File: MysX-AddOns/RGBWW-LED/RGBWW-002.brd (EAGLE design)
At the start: 47 x 53 mm, 14 parts

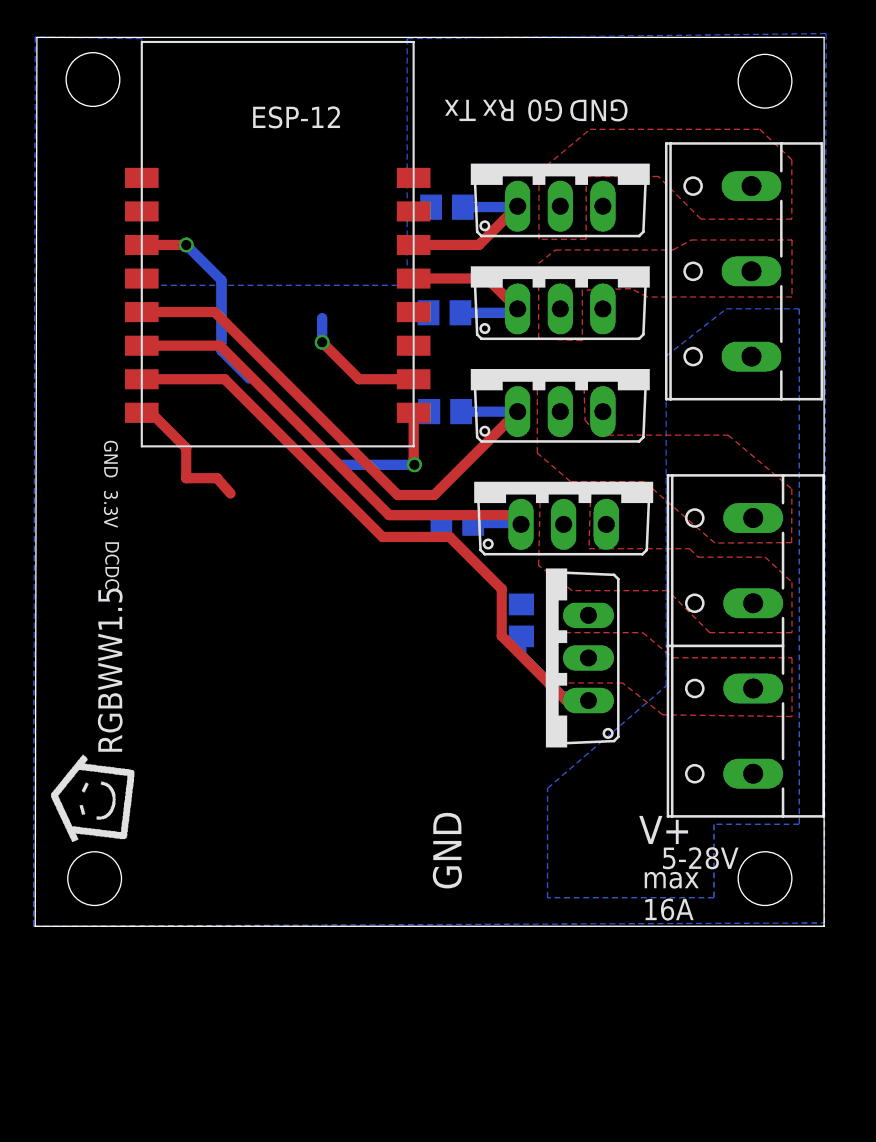
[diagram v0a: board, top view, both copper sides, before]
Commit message: AddOns
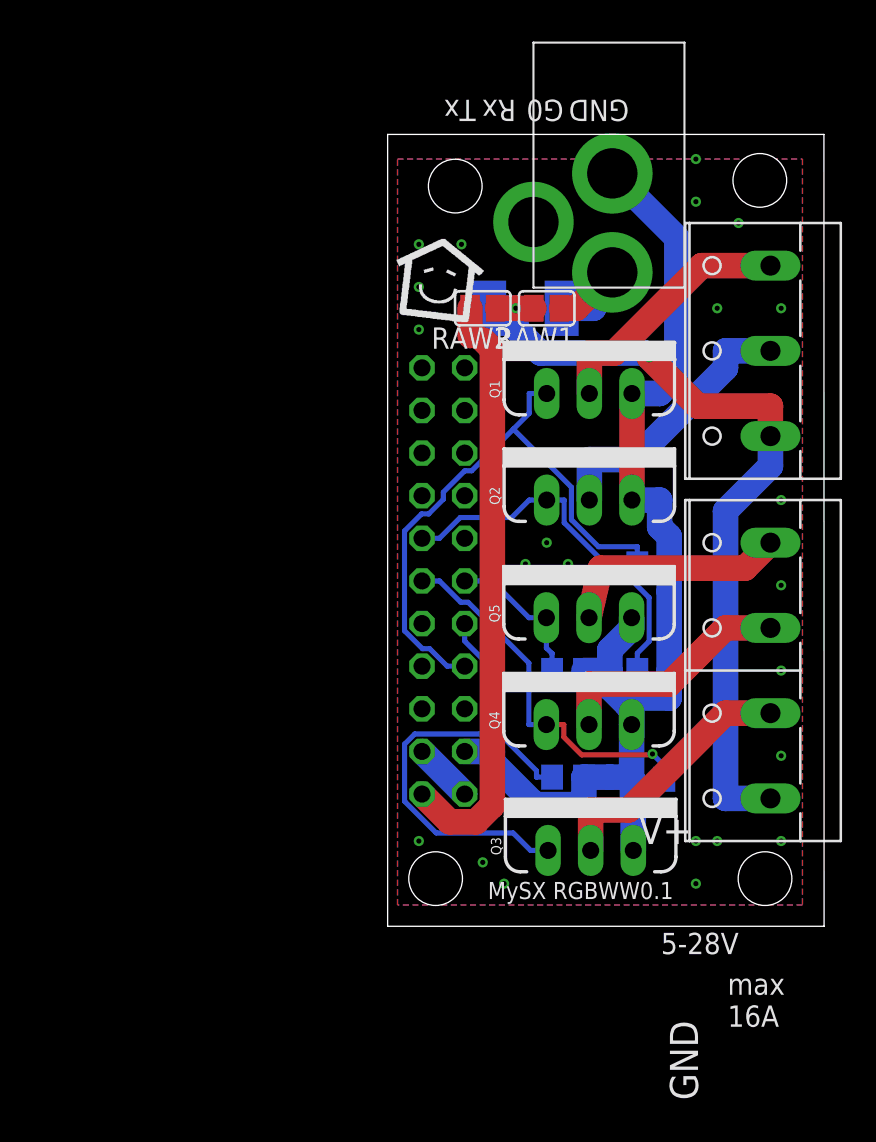
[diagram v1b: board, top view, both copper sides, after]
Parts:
- removed ESP-12: ESP8266_ESP-12, ESP8266-ESP12:ESP8266-ESP12
- removed IRLZ44N-B, IRLZ44N-CW, IRLZ44N-G, IRLZ44N-R, IRLZ44N-WW: (no value), PAsystem:TO220AV
- removed U$1: (no value), fhem.logo:LOGO
- added F2: 1812L, ptc-littlefuse:1812L
- added Q1, Q2, Q3, Q4, Q5: 60V/32A/35mΩ, SparkFun-DiscreteSemi:TO220V
- added RAW1, RAW2: (no value), jumper:SJ
- added SV2: (no value), con-Pinheader:MA11-2
- added U$2: (no value), fhem.logo:LOGO
- added U$3: 2.1MMJACKTHM, adafruit:PJ-102A
- moved R2 24.7 mm to (36.8, 15.2)
- moved R1 24.6 mm to (36.8, 21.6), turned to 0 degrees
- moved R3 23.0 mm to (31.8, 8.89)
- moved R4 19.1 mm to (36.5, 8.76), turned to 180 degrees
- moved W 4.87 mm to (43.2, 34.3)
- moved R5 4.08 mm to (31.8, 15.2), turned to 0 degrees
- moved RGB 1.79 mm to (43.2, 15.2)
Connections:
- removed net +3V3: ESP-12.16
- removed net N$2: ESP-12.11
- removed net N$7: ESP-12.2
- removed net RGB-B: ESP-12.13, IRLZ44N-B.B, R3.1
- removed net RGB-B-OUT: IRLZ44N-B.C, RGB.4
- removed net RGB-CW: ESP-12.5, IRLZ44N-CW.B, R2.1
- removed net RGB-CW-OUT: IRLZ44N-CW.C, W.2
- removed net RGB-G: ESP-12.14, IRLZ44N-G.B, R4.1
- removed net RGB-G-OUT: IRLZ44N-G.C, RGB.3
- removed net RGB-R: ESP-12.15, IRLZ44N-R.B, R5.1
- removed net RGB-R-OUT: IRLZ44N-R.C, RGB.2
- removed net RGB-WW: ESP-12.6, IRLZ44N-WW.B, R1.2
- new net A0: Q1.1, R1.2, SV2.8
- new net A1: SV2.14
- new net A2: SV2.16
- new net A3: SV2.15
- new net D10_SS: SV2.20
- new net D11_MOSI: SV2.17
- new net D12_MISO: SV2.18
- new net D13_SCK: SV2.19
- new net D2: SV2.9
- new net D3: Q3.1, R3.2, SV2.10
- new net D5: Q4.1, R4.2, SV2.11
- new net D6: Q5.1, R5.2, SV2.12
- new net D7: SV2.22
- new net D8: Q2.1, R2.2, SV2.13
- new net D9: SV2.21
- new net RESET: SV2.7
- new net RGB-WW-OUT1: Q2.2, W.2
- new net RGB-WW-OUT2: Q3.2, RGB.2
- new net RGB-WW-OUT3: Q4.2, RGB.3
- new net RGB-WW-OUT4: Q5.2, RGB.4
- new net RX0: SV2.6
- new net TX1: SV2.5
- new net UREG: RAW2.2, SV2.1
- new net VCC: SV2.2, SV2.3
- new net VIN: F2.P$2, RAW1.1, U$3.TIP
- net +12V: now also F2.P$1, RAW1.2, RAW2.1
- net GND: now also Q1.3, Q2.3, Q3.3, Q4.3, Q5.3, R2.1, R3.1, R4.1, R5.1, SV2.4, U$3.RING; no longer ESP-12.1, IRLZ44N-B.E, IRLZ44N-CW.E, IRLZ44N-G.E, IRLZ44N-R.E, IRLZ44N-WW.E, R2.2, R3.2, R4.2, R5.2
- net RGB-WW-OUT: now also Q1.2; no longer IRLZ44N-WW.C
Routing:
- net GND: track 7.56 -> 69.2 mm, vias 1 -> 23
- net +12V: track 0.00 -> 49.3 mm, vias 0 -> 2
- net RGB-R: track 42.5 -> 0.00 mm
- net UREG: track 0.00 -> 35.8 mm
- net A0: track 0.00 -> 35.7 mm
- net RGB-B: track 32.3 -> 0.00 mm
- net D3: track 0.00 -> 30.6 mm
- net RGB-G: track 29.9 -> 0.00 mm
- net D5: track 0.00 -> 22.6 mm, vias 0 -> 1
- net D8: track 0.00 -> 22.3 mm
- net RGB-WW-OUT1: track 0.00 -> 16.5 mm
- net RGB-WW-OUT2: track 0.00 -> 15.5 mm
- net RGB-WW-OUT: track 0.00 -> 15.4 mm
- net RGB-WW-OUT3: track 0.00 -> 14.6 mm
- net RGB-WW-OUT4: track 0.00 -> 13.8 mm
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- added copper zone on layer 1, net GND
- removed copper zone on layer 16, net +12V
- removed copper zone on layer 1, net RGB-B-OUT
- removed copper zone on layer 1, net RGB-CW-OUT
- removed copper zone on layer 1, net RGB-G-OUT
- removed copper zone on layer 1, net RGB-R-OUT
- removed copper zone on layer 1, net RGB-WW-OUT
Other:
- board size 47 x 53 mm -> 26 x 47.2 mm
- board text added: "MySX RGBWW0.1"
- board text removed: "3.3V"
- board text removed: "RGBWW1.5"
